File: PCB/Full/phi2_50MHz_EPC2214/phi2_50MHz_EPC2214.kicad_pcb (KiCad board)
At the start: 2 copper layers, 70 x 70 mm, 63 parts, among them Q1 EPC2214, U1 TPS563203, U3 NC7WZ04, U4 TLV3501, U5 NC7WZ04, U6 NC7WZ04, U7 NC7WZ04

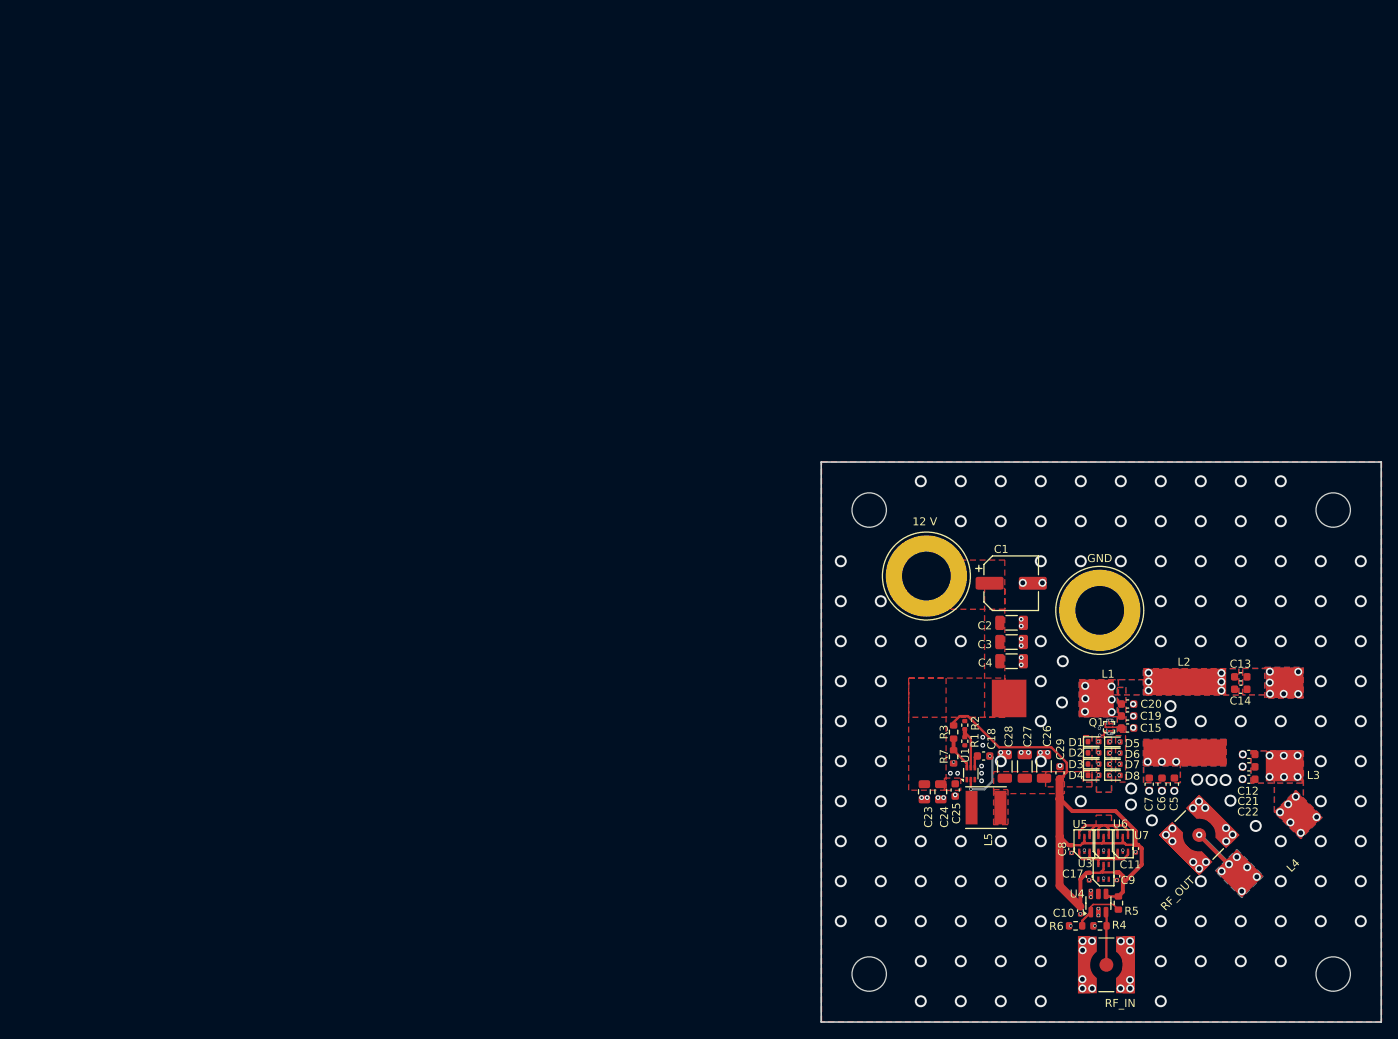
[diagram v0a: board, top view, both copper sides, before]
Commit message: gerbers and rev1 board sent out
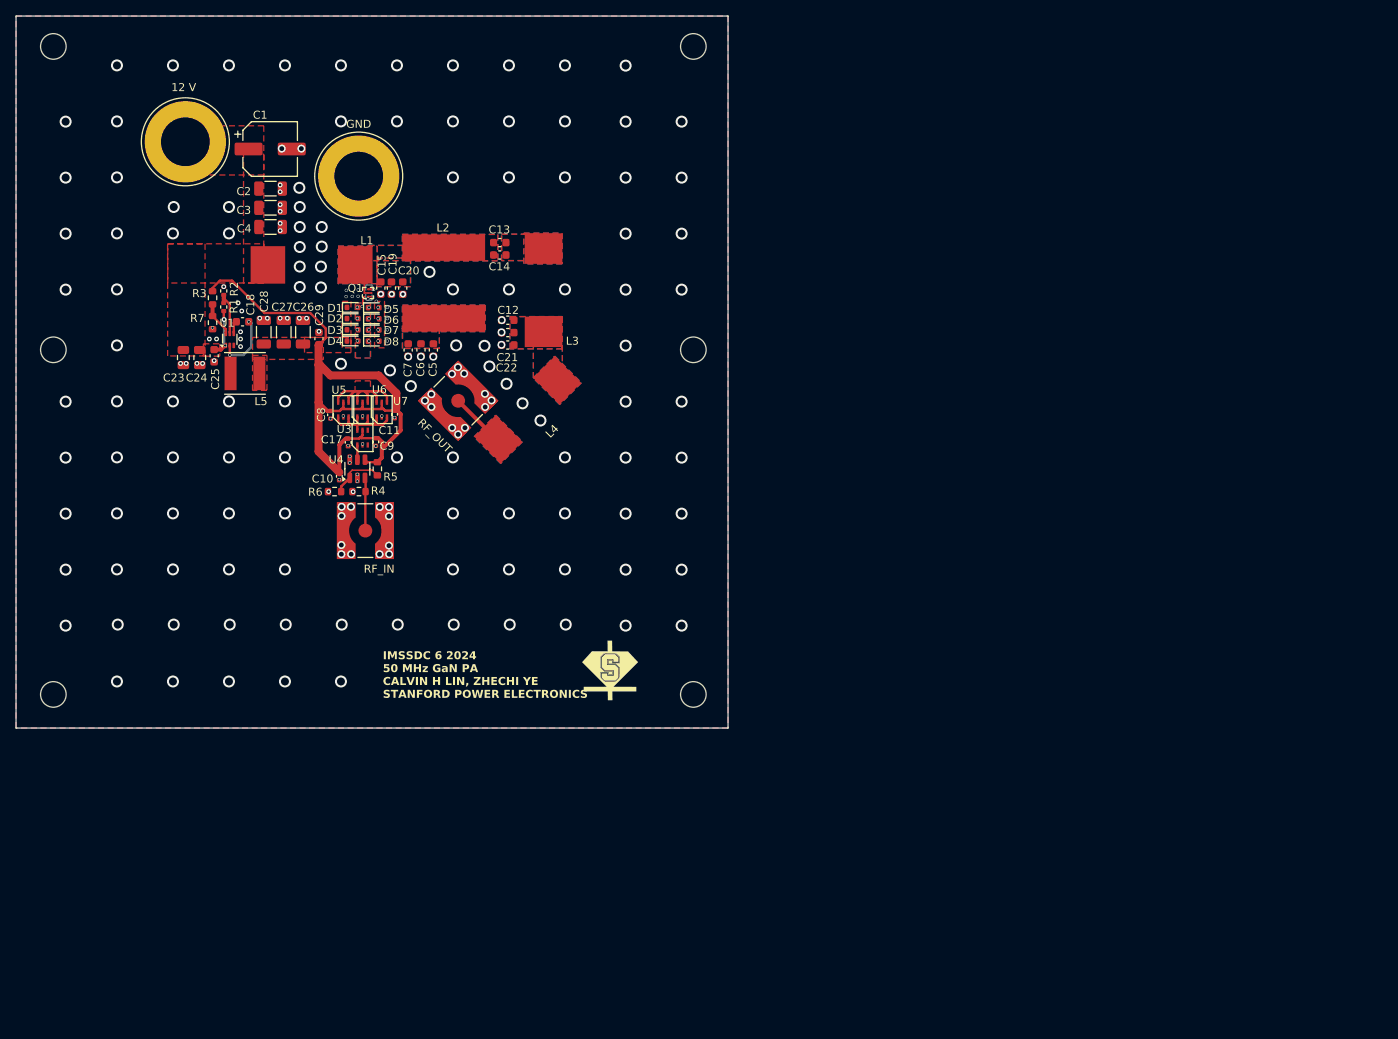
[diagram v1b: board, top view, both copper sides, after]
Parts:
- removed the REF** at (164.7, 61.8)
- removed the REF** at (106.7, 61.8)
- removed the REF** at (164.7, 119.8)
- removed the REF** at (106.7, 119.8)
- added G***: LOGO, Logo:superlab_logo, F.Cu at (74.3, 81.8)
- added REF**: MountingHole_3.2mm_M3_DIN965, MountingHole:MountingHole_3.2mm_M3_DIN965, F.Cu at (4.67, 84.8)
- added REF**: MountingHole_3.2mm_M3_DIN965, MountingHole:MountingHole_3.2mm_M3_DIN965, F.Cu at (84.7, 41.7)
- added REF**: MountingHole_3.2mm_M3_DIN965, MountingHole:MountingHole_3.2mm_M3_DIN965, F.Cu at (84.7, 3.80)
- added REF**: MountingHole_3.2mm_M3_DIN965, MountingHole:MountingHole_3.2mm_M3_DIN965, F.Cu at (4.67, 3.80)
- added REF**: MountingHole_3.2mm_M3_DIN965, MountingHole:MountingHole_3.2mm_M3_DIN965, F.Cu at (84.7, 84.8)
- added REF**: MountingHole_3.2mm_M3_DIN965, MountingHole:MountingHole_3.2mm_M3_DIN965, F.Cu at (4.67, 41.7)
- moved C15 108.3 mm to (45.6, 34.0), turned to -90 degrees
- moved C1 107.4 mm to (31.8, 16.6)
- moved C10 107.4 mm to (40.4, 57.5)
- moved C25 107.4 mm to (24.8, 42.5)
- moved C5 107.4 mm to (52.2, 41.7)
- moved R5 107.4 mm to (45.2, 56.6)
- moved RF_IN 107.4 mm to (43.7, 64.3)
- moved U4 107.4 mm to (42.7, 56.6)
- moved U5 107.4 mm to (40.9, 49.2)
- moved 12 V 107.4 mm to (21.2, 15.7)
- moved C11 107.4 mm to (47.3, 49.8)
- moved C12 107.4 mm to (61.5, 38.0)
- moved C13 107.4 mm to (60.5, 28.3)
- moved C14 107.4 mm to (60.5, 29.9)
- moved C17 107.4 mm to (41.5, 53.3)
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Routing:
- net +12V: track 0.19 -> 6.13 mm, vias 0 -> 2
- net Net-(J2-In): track 10.6 -> 5.35 mm, vias 7 -> 0
- net +5V: track 83.7 -> 85.7 mm
- net Net-(U3-A1): track 0.00 -> 1.98 mm
- net GND: track 1.68 -> 1.91 mm, vias 212 -> 210
- net /D: track 2.38 -> 2.61 mm, vias 12 -> 0
- net Net-(C5-Pad1): vias 3 -> 0
- net Net-(C13-Pad2): vias 6 -> 0
- net Net-(C12-Pad1): vias 12 -> 0
- added copper zone on F.Cu, net Net-(J2-In)
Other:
- board size 70 x 70 mm -> 89 x 89 mm
- board text added: "IMSSDC 6 2024 50 MHz GaN PA CALVIN H LIN, ZHECHI YE STANFORD POWER ELECTRONICS"
- board text removed: "IMSSDC 6 50 MHz GaN PA CALVIN H LIN, ZHECHI YE"
